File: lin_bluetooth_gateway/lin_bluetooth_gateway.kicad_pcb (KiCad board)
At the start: 2 copper layers, 22.8 x 14.5 mm, 9 parts, among them P1 CONN_01X01, P2 CONN_01X01, P3 CONN_01X01, P4 CONN_01X03, U1 MCP2050, U2 BL652

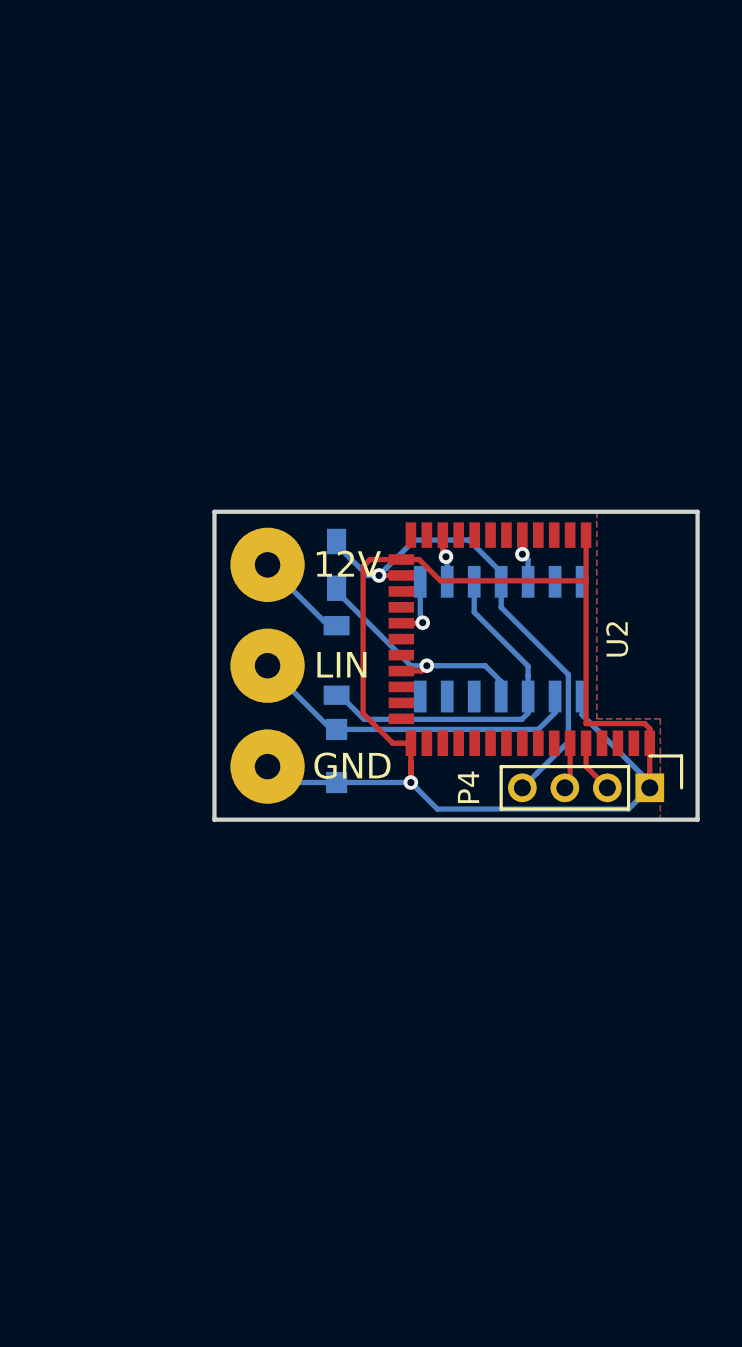
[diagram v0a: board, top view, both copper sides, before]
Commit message: lin_bluetooth_gateway rev2
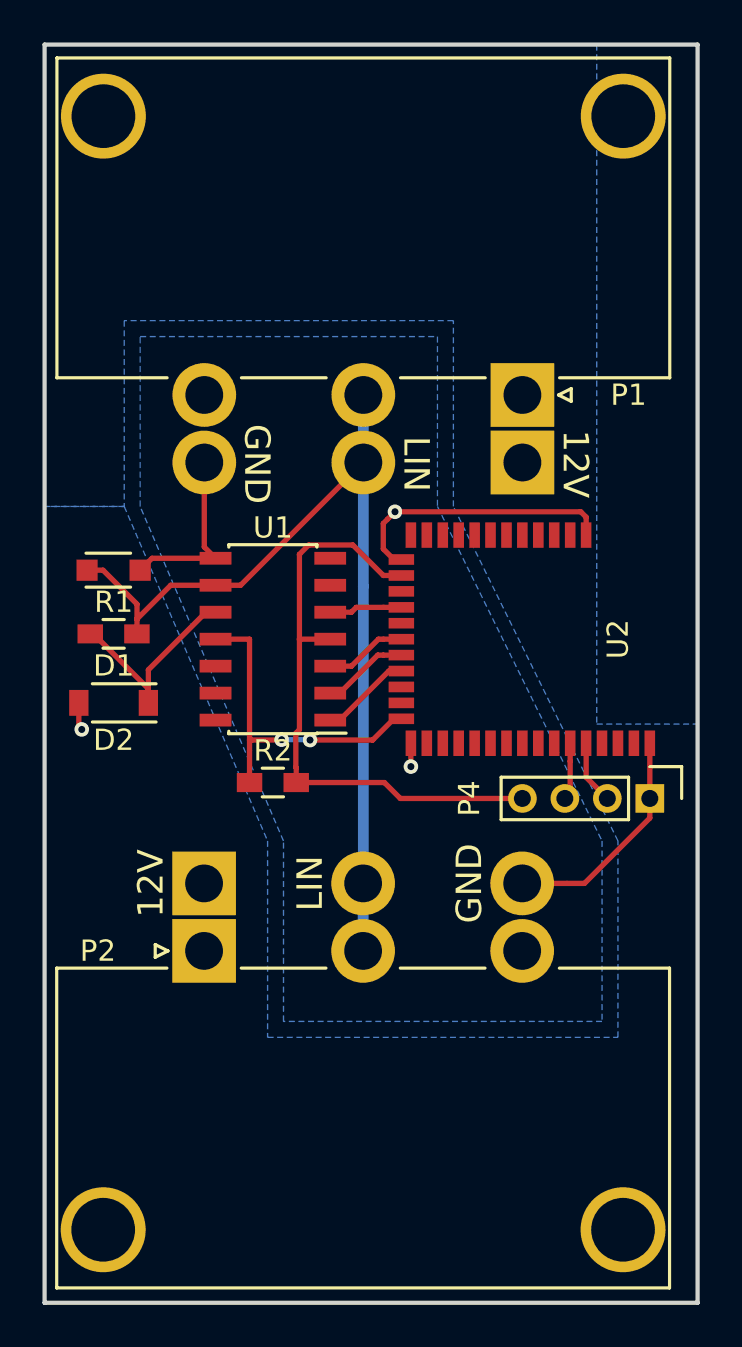
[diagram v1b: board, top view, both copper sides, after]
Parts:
- removed P3: CONN_01X01, Wire_Pads:SolderWirePad_single_1-2mmDrill
- added R1: 10k, Resistors_SMD:R_0603_HandSoldering, F.Cu at (136.8, 102.2)
- D1, D2, R2, U1: moved to F.Cu
- P1, P2: value CONN_01X01 -> MOLEX-0431603103; footprint Wire_Pads:SolderWirePad_single_1-2mmDrill -> Connectors_Molex:Molex_Sabre_43160-XX03_03x7.49mm_Angled_BoardLock
- moved P1 21.2 mm to (156.0, 91.0), turned to 180 degrees
- moved P2 13.8 mm to (141.0, 117.2)
- moved D1 13.7 mm to (136.8, 99.2), turned to 0 degrees
- moved U1 10.8 mm to (144.2, 102.5), turned to 180 degrees
- moved D2 10.7 mm to (136.8, 105.5), turned to 180 degrees
- moved R2 10.7 mm to (144.2, 109.2), turned to 180 degrees
- moved P4 0.50 mm to (162.0, 110.0)
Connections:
- D2 pad 2: Net-(D2-Pad2) -> /12V_UNPROTECTED
- P1 pad 1: GND -> /12V_UNPROTECTED
- P2 pad 1: Net-(D1-Pad1) -> /12V_UNPROTECTED
- R2 pad 2: Net-(R2-Pad2) -> /FAULT
- U1 pad 1: Net-(U1-Pad1) -> /VBAT_RATIO
- U1 pad 11: Net-(R2-Pad2) -> /FAULT
- U1 pad 2: Net-(U1-Pad2) -> /RXD
- U1 pad 3: +12V -> /CS/LWAKE
- U1 pad 5: Net-(U1-Pad5) -> /TXD
- U2 pad 17: (no net) -> /FAULT
- U2 pad 20: Net-(R2-Pad2) -> /VBAT_RATIO
- U2 pad 21: (no net) -> /RXD
- U2 pad 22: (no net) -> /CS/LWAKE
- U2 pad 23: Net-(U1-Pad1) -> (no net)
- U2 pad 24: (no net) -> /TXD
- U2 pad 30: Net-(U1-Pad2) -> (no net)
- U2 pad 35: Net-(U1-Pad5) -> (no net)
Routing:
- net GND: track 64.0 -> 33.7 mm, vias 1 -> 2
- net Net-(D1-Pad1): track 15.9 -> 44.3 mm
- net /FAULT: track 0.00 -> 15.9 mm, vias 0 -> 2
- net Net-(R2-Pad2): track 11.7 -> 0.00 mm, vias 1 -> 0
- net +12V: track 16.8 -> 10.3 mm
- net +3V3: track 23.6 -> 28.8 mm, vias 1 -> 0
- net Net-(D2-Pad2): track 4.44 -> 0.00 mm
- net /VBAT_RATIO: track 0.00 -> 4.31 mm
- net /RXD: track 0.00 -> 4.09 mm
- net /CS/LWAKE: track 0.00 -> 3.88 mm
- net /TXD: track 0.00 -> 3.45 mm
- net Net-(U1-Pad1): track 2.99 -> 0.00 mm, vias 1 -> 0
- net Net-(U1-Pad5): track 2.31 -> 0.00 mm, vias 1 -> 0
- net Net-(U1-Pad2): track 2.29 -> 0.00 mm, vias 1 -> 0
- net /12V_UNPROTECTED: track 0.00 -> 1.31 mm, vias 0 -> 1
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- added copper zone on B.Cu, net /12V_UNPROTECTED
- removed copper zone on F.Cu, net GND
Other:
- board size 22.8 x 14.5 mm -> 30.8 x 59.2 mm
- board text added: "LIN<->BLE Gateway Rev 2, Nov 2016 Cedric Priscal"
- board text removed: "3V"
- board text removed: "CK"
- board text removed: "GD"
- board text removed: "IO"
- board text removed: "LIN<->BLE Gateway"
